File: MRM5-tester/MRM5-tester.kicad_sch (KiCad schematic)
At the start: 0 parts

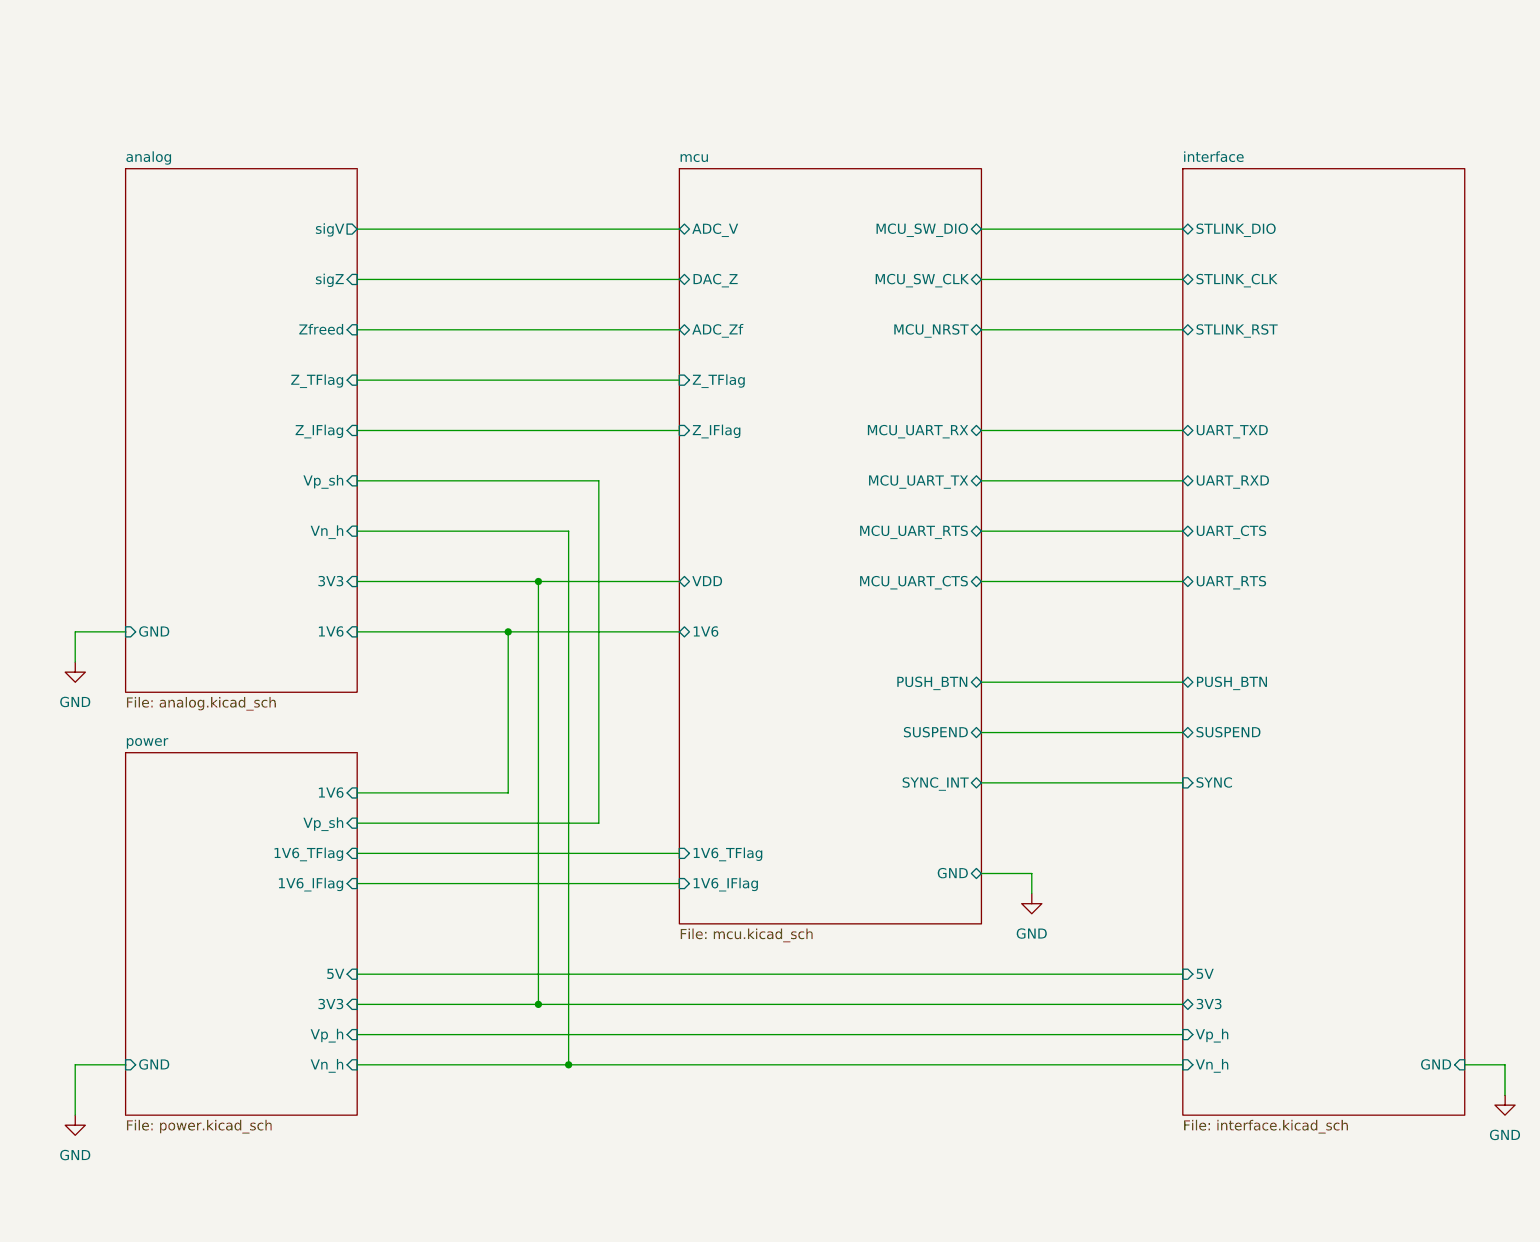
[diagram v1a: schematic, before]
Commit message: tester pcb updated
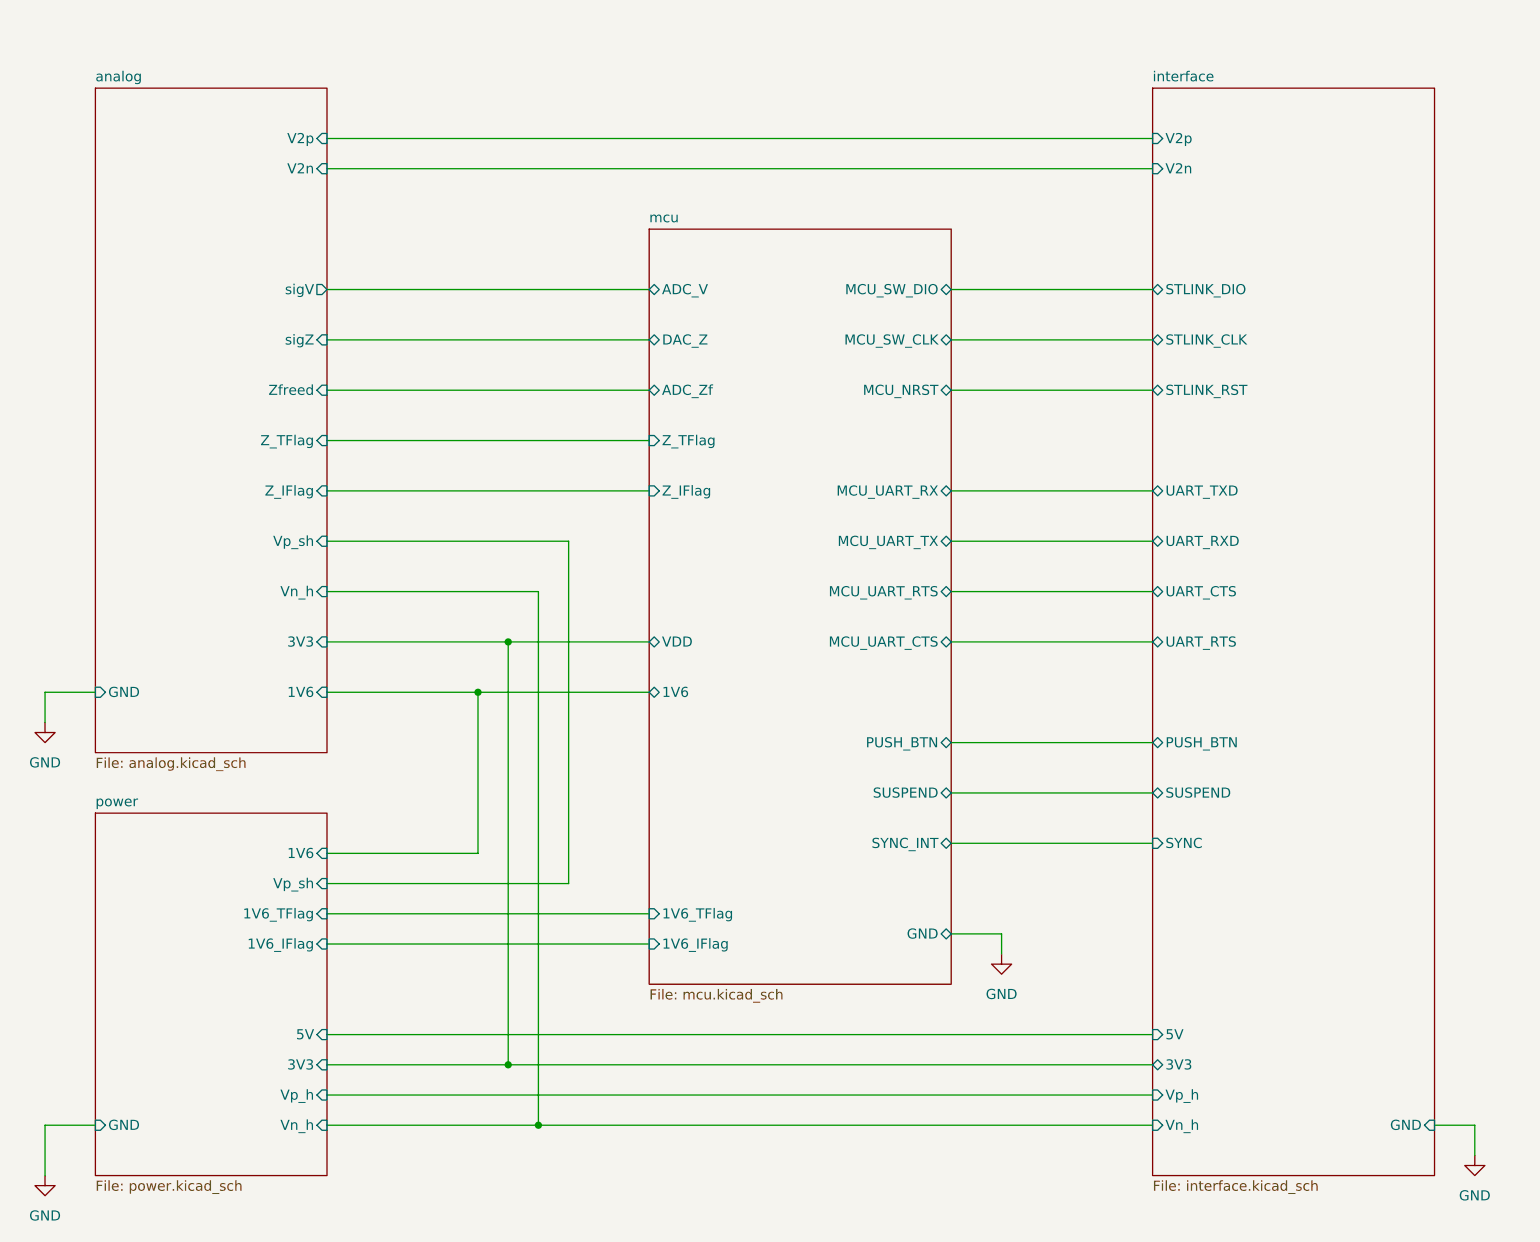
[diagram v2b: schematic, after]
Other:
- sheet analog ports: added V2n, V2p; removed none
- sheet interface ports: added V2n, V2p; removed none

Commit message: 케이스에 마춰서 제작 중
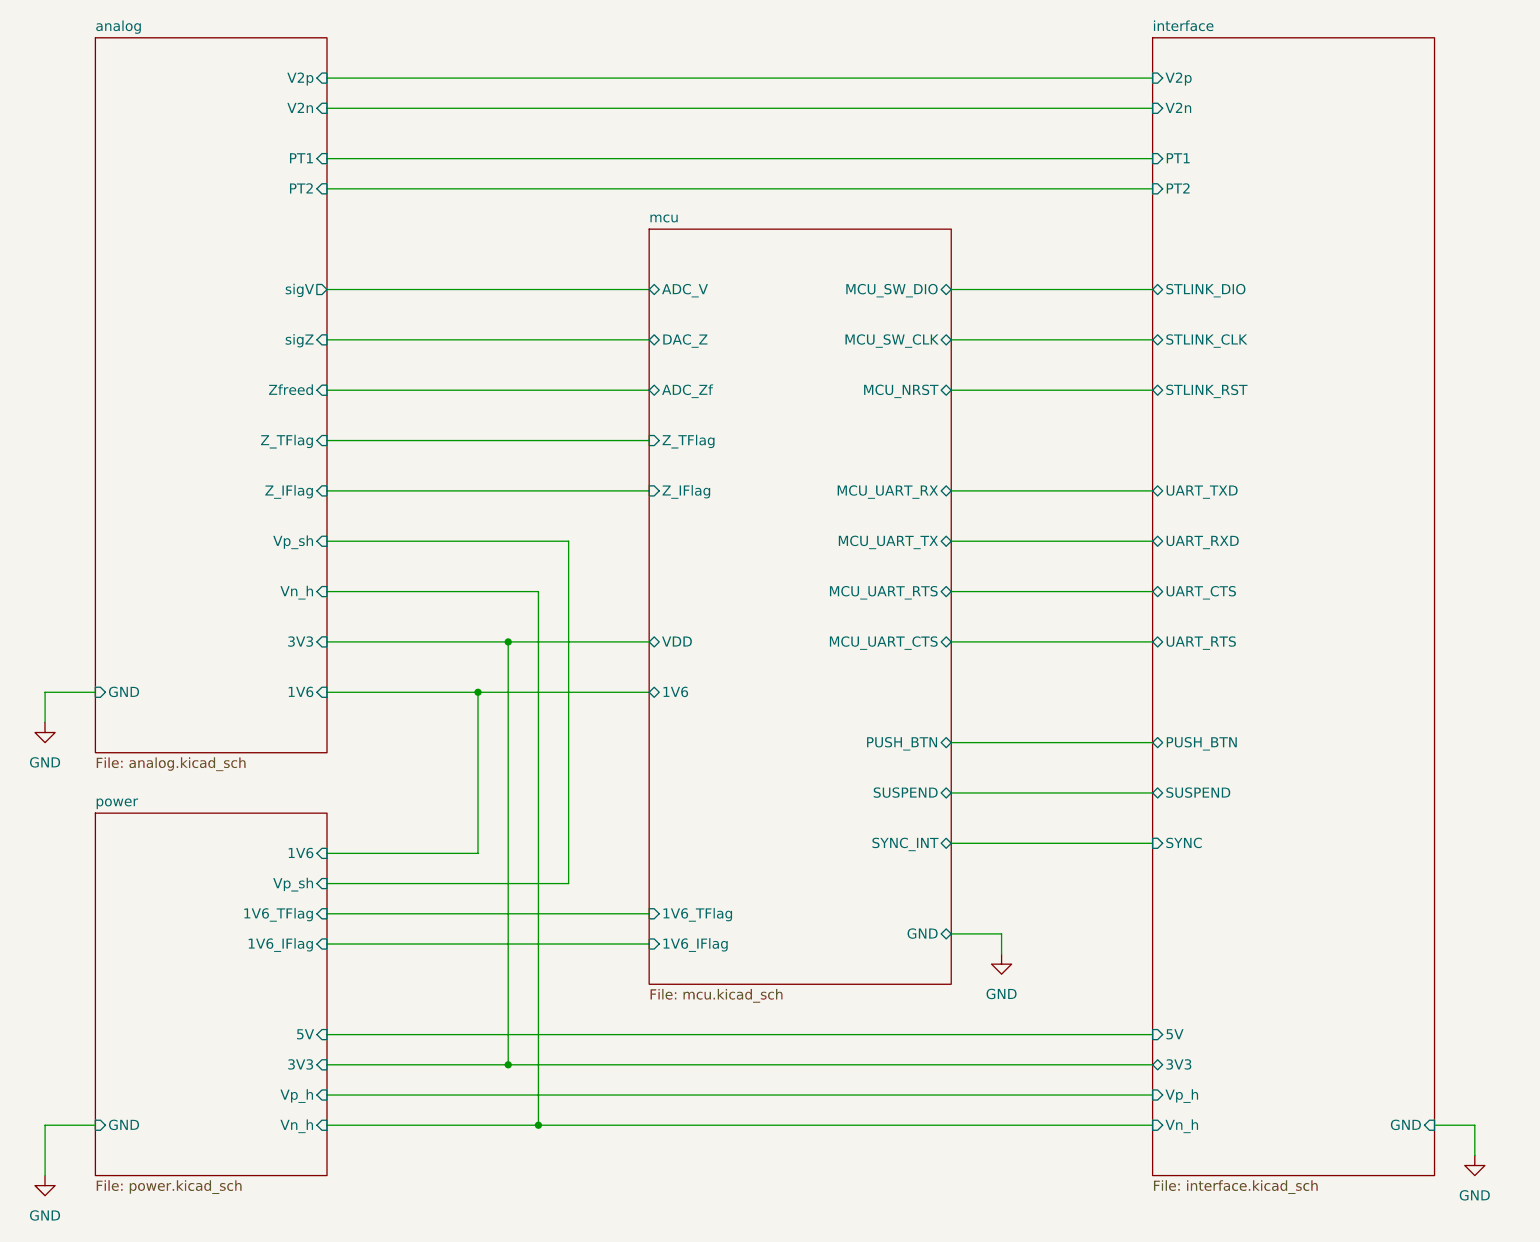
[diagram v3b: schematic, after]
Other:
- sheet analog ports: added PT1, PT2; removed none
- sheet interface ports: added PT1, PT2; removed none
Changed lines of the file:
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@@
+	(wire
+		(pts
+			(xy 90.17 31.75) (xy 194.31 31.75)
+		)
+		(stroke
+			(width 0)
+			(type default)
+		)
+	)
 	(wire
 		(pts
@@
 	(wire
 		(pts
-			(xy 90.17 29.21) (xy 194.31 29.21)
+			(xy 90.17 21.59) (xy 194.31 21.59)
 		)
 		(stroke
@@
 	(wire
 		(pts
-			(xy 90.17 33.02) (xy 194.31 33.02)
+			(xy 90.17 25.4) (xy 194.31 25.4)
 		)
 		(stroke
@@
 		(pts
 			(xy 90.17 73.66) (xy 130.81 73.66)
+		)
+		(stroke
+			(width 0)
+			(type default)
+		)
+	)
+	(wire
+		(pts
+			(xy 90.17 35.56) (xy 194.31 35.56)
 		)
 		(stroke
@@
 	)
 	(sheet
-		(at 194.31 22.86)
-		(size 35.56 137.16)
+		(at 194.31 16.51)
+		(size 35.56 143.51)
 		(fields_autoplaced yes)
 		(stroke
@@
 		)
 		(property "Sheetname" "interface"
-			(at 194.31 22.1484 0)
+			(at 194.31 15.7984 0)
 			(effects
 				(font
@@
 		)
 		(pin "V2n" input
-			(at 194.31 33.02 180)
+			(at 194.31 25.4 180)
 			(effects
 				(font
@@
 		)
 		(pin "V2p" input
-			(at 194.31 29.21 180)
+			(at 194.31 21.59 180)
+			(effects
+				(font
+					(size 1.27 1.27)
+				)
+				(justify left)
+			)
+		)
+		(pin "PT2" input
+			(at 194.31 35.56 180)
+			(effects
+				(font
+					(size 1.27 1.27)
+				)
+				(justify left)
+			)
+		)
+		(pin "PT1" input
+			(at 194.31 31.75 180)
 			(effects
 				(font
@@
 	)
 	(sheet
-		(at 60.96 22.86)
-		(size 29.21 83.82)
+		(at 60.96 16.51)
+		(size 29.21 90.17)
 		(fields_autoplaced yes)
 		(stroke
@@
 		)
 		(property "Sheetname" "analog"
-			(at 60.96 22.1484 0)
+			(at 60.96 15.7984 0)
 			(effects
 				(font
@@
 		)
 		(pin "V2p" input
-			(at 90.17 29.21 0)
+			(at 90.17 21.59 0)
 			(effects
 				(font
@@
 		)
 		(pin "V2n" input
-			(at 90.17 33.02 0)
-			(effects
-				(font
+			(at 90.17 25.4 0)
+			(effects
+				(font
+					(size 1.27 1.27)
+				)
+				(justify right)
+			)
+		)
+		(pin "PT1" input
+			(at 90.17 31.75 0)
+			(effects
+				(font
+					(size 1.27 1.27)
+				)
+				(justify right)
+			)
+		)
+		(pin "PT2" input
+			(at 90.17 35.56 0)
+			(effects
+				(font

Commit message: 1차 마감
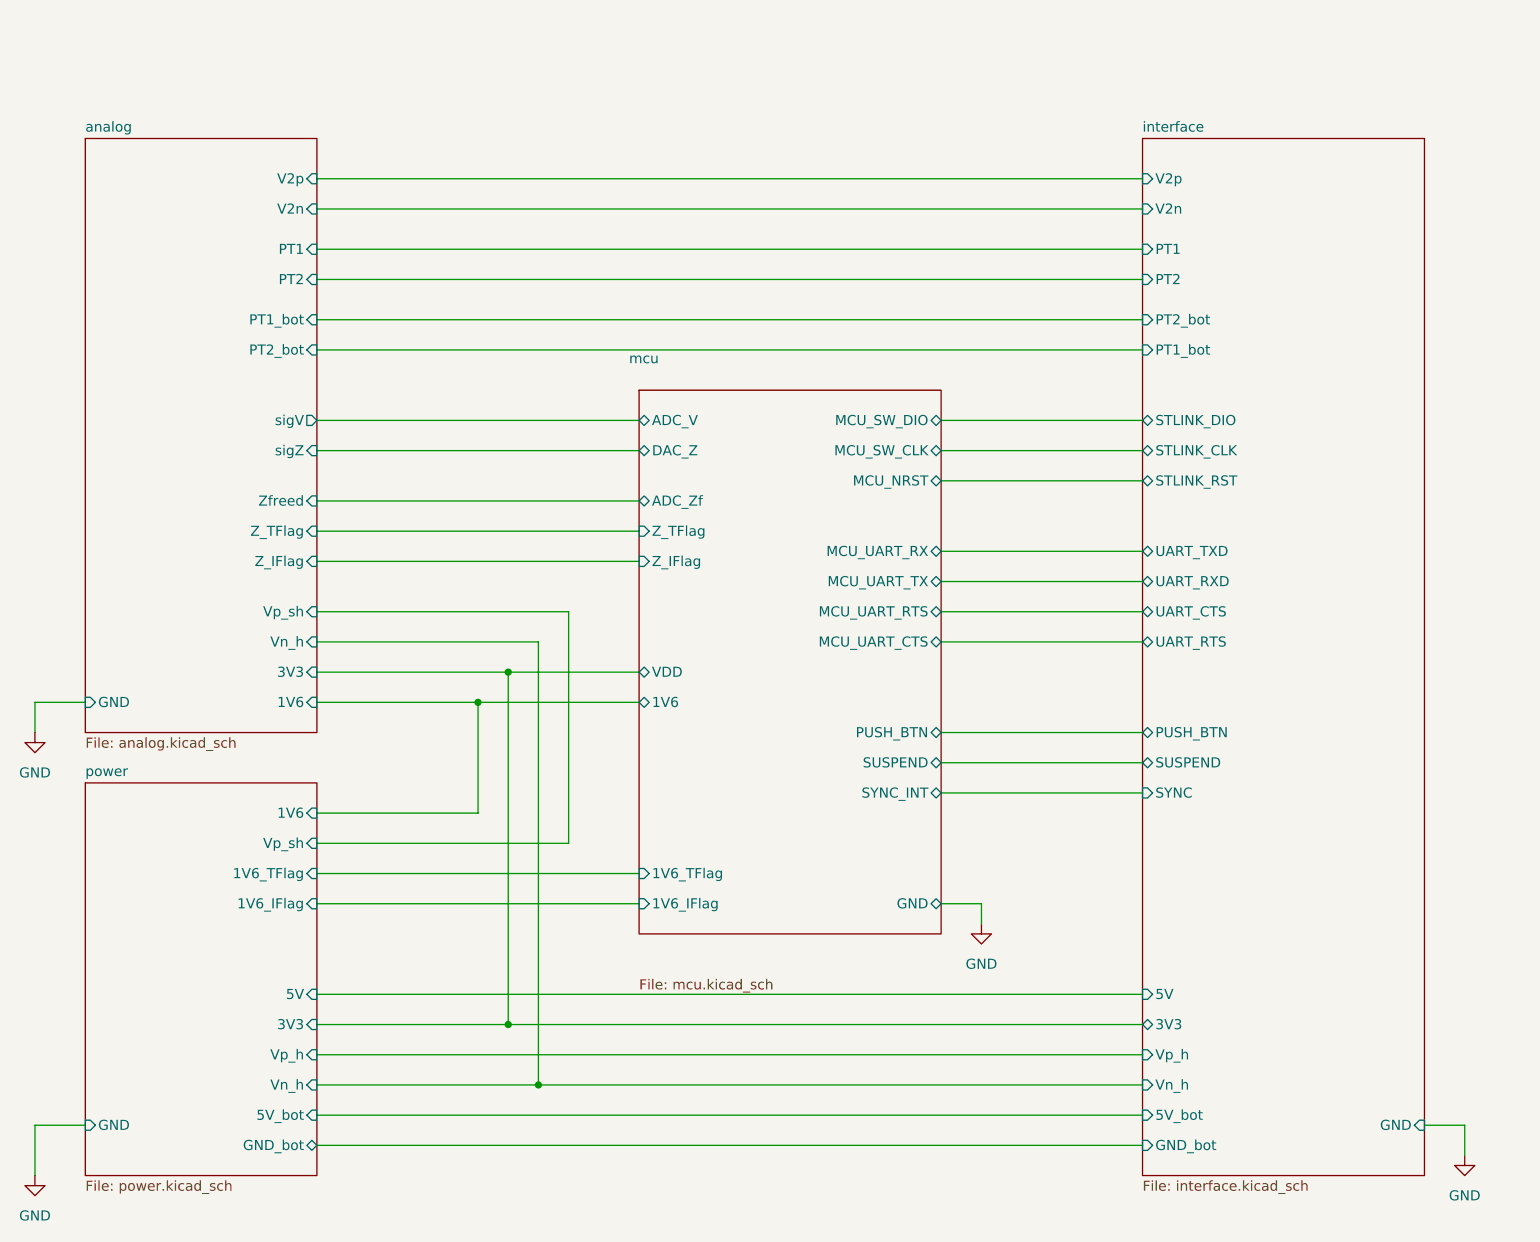
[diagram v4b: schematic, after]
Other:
- sheet analog ports: added PT1_bot, PT2_bot; removed none
- sheet interface ports: added 5V_bot, GND_bot, PT1_bot, PT2_bot; removed none
- sheet power ports: added 5V_bot, GND_bot; removed none
